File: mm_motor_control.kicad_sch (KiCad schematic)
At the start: 0 parts

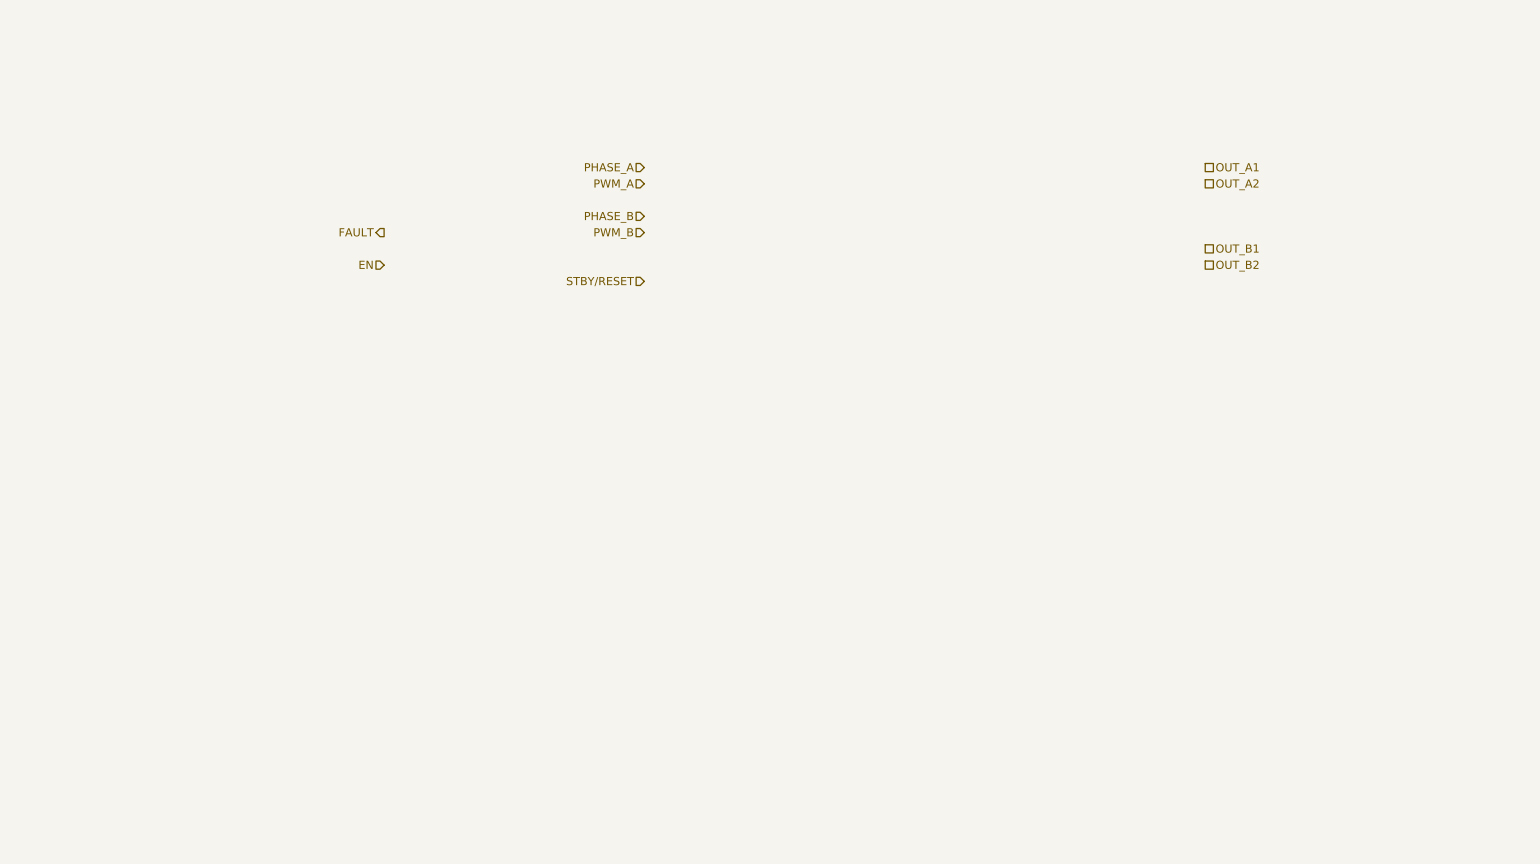
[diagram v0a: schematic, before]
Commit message: fin tp2
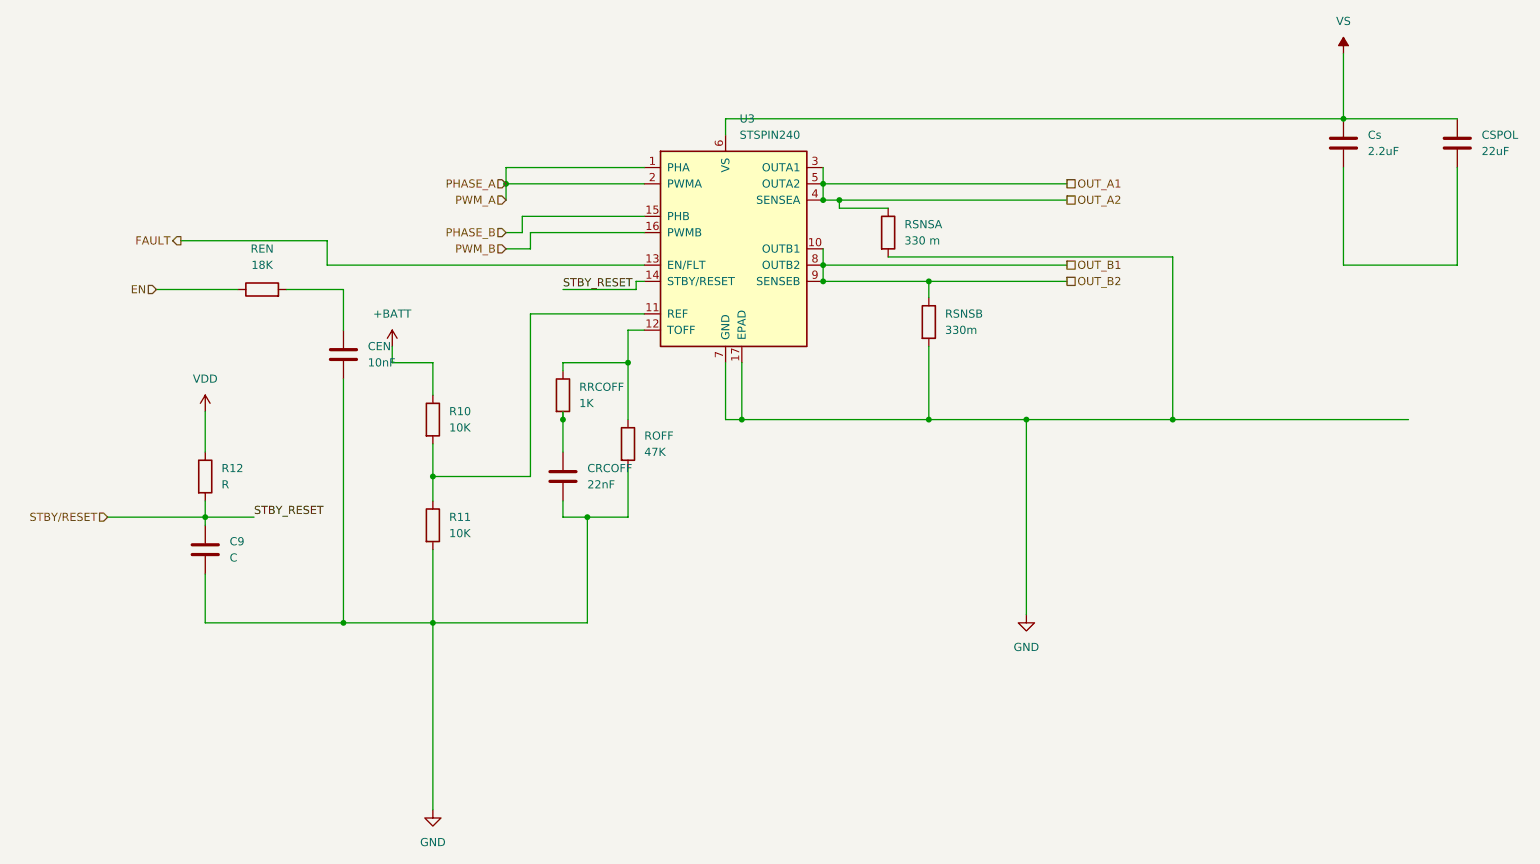
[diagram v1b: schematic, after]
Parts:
- added C9: C, symbol Device:C
- added CEN: 10nF, symbol Device:C
- added CRCOFF: 22nF, symbol Device:C
- added CSPOL: 22uF, symbol Device:C
- added Cs: 2.2uF, symbol Device:C
- added R10, R11: 10K, symbol Device:R
- added R12: R, symbol Device:R
- added REN: 18K, symbol Device:R
- added ROFF: 47K, symbol Device:R
- added RRCOFF: 1K, symbol Device:R
- added RSNSA: 330 m, symbol Device:R
- added RSNSB: 330m, symbol Device:R
- added U3: STSPIN240, Package_DFN_QFN:VQFN-16-1EP_3x3mm_P0.5mm_EP1.8x1.8mm, symbol Driver_Motor:STSPIN240
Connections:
- net EN: now also REN.1
- net FAULT: now also U3.13 (EN/FLT)
- net OUT_A1: now also RSNSA.1, U3.3 (OUTA1), U3.4 (SENSEA), U3.5 (OUTA2)
- net OUT_B1: now also RSNSB.1, U3.10 (OUTB1), U3.8 (OUTB2), U3.9 (SENSEB)
- net PHASE_A: now also U3.1 (PHA), U3.2 (PWMA)
- net PHASE_B: now also U3.15 (PHB)
- net PWM_B: now also U3.16 (PWMB)
- net STBY/RESET: now also C9.1, R12.2, U3.14 (STBY/RESET)
- new net: CEN.1, REN.2
- new net: CSPOL.2, Cs.2
- new net: ROFF.1, RRCOFF.1, U3.12 (TOFF)
- new net: R10.2, R11.1, U3.11 (REF)
- new net: CRCOFF.1, RRCOFF.2
- new net +BATT: R10.1
- new net GND: C9.2, CEN.2, CRCOFF.2, R11.2, ROFF.2, RSNSA.2, RSNSB.2, U3.17 (EPAD), U3.7 (GND)
- new net VDD: R12.1
- new net VS: CSPOL.1, Cs.1, U3.6 (VS)
